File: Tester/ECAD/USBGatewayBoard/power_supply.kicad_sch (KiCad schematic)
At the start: 2 parts, among them J2 Barrel_Jack, J8 Barrel_Jack_MountingPin

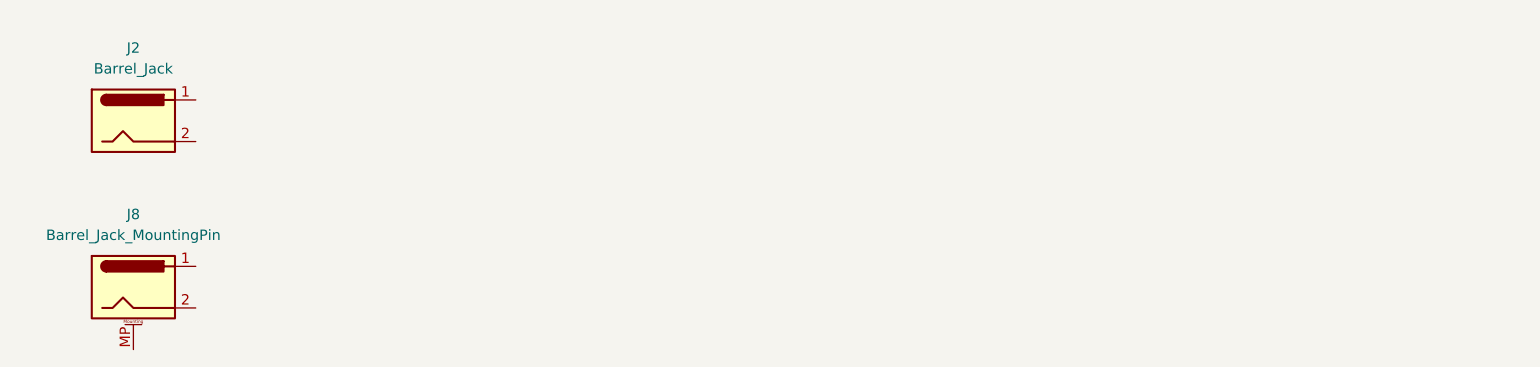
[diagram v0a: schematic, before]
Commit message: Progressed ECAD
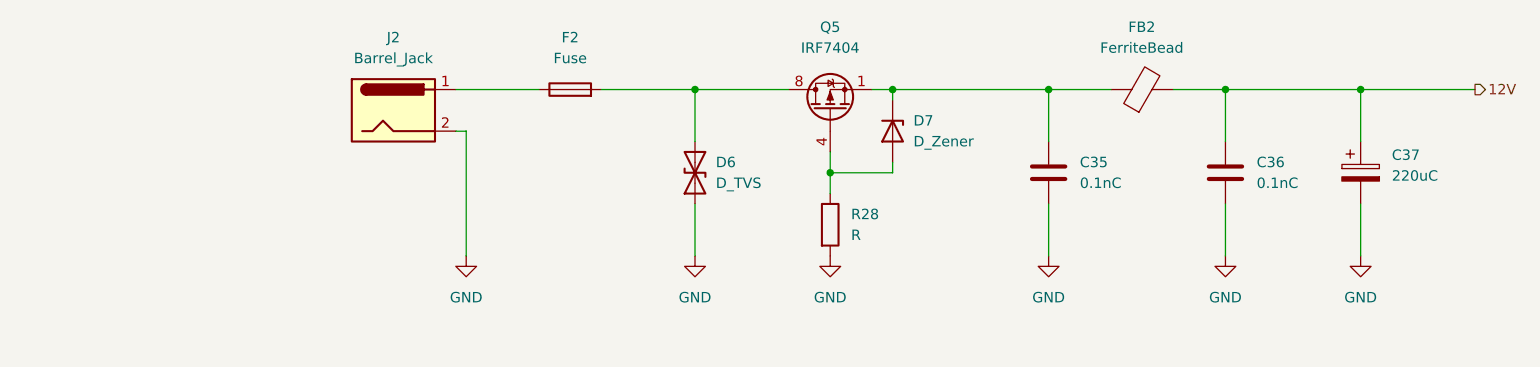
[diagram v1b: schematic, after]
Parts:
- removed J8: Barrel_Jack_MountingPin, Connector_BarrelJack:BarrelJack_CUI_PJ-063AH_Horizontal, symbol Connector:Barrel_Jack_MountingPin
- added C35, C36: 0.1nC, Capacitor_SMD:C_0805_2012Metric_Pad1.18x1.45mm_HandSolder, symbol Device:C
- added C37: 220uC, Capacitor_THT:CP_Radial_D8.0mm_P3.50mm, symbol Device:C_Polarized
- added D6: D_TVS, Diode_SMD:D_SMA, symbol Device:D_TVS
- added D7: D_Zener, symbol Device:D_Zener
- added F2: Fuse, symbol Device:Fuse
- added FB2: FerriteBead, Inductor_SMD:L_1806_4516Metric_Pad1.45x1.90mm_HandSolder, symbol Device:FerriteBead
- added Q5: IRF7404, Package_SO:SOIC-8_3.9x4.9mm_P1.27mm, symbol Transistor_FET:IRF7404
- added R28: R, Resistor_SMD:R_0805_2012Metric_Pad1.20x1.40mm_HandSolder, symbol Device:R
- J2: Manufacturer Part Number (none) -> DC-042C-W-2.5
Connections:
- net at J2.1: now also F2.1
- net GND: now reaches J2.2
- net GND: now also C35.2, C36.2, C37.2, D6.1 (A1), R28.2
- new net: C35.1, D7.1 (K), FB2.1, Q5.1 (S), Q5.2 (S), Q5.3 (S)
- new net: D6.2 (A2), F2.2, Q5.5 (D), Q5.6 (D), Q5.7 (D), Q5.8 (D)
- new net: D7.2 (A), Q5.4 (G), R28.1
- new net 12V: C36.1, C37.1, FB2.2
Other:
- moved on the sheet: J2
